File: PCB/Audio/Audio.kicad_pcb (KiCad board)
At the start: 2 copper layers, 70 x 70 mm, 54 parts, among them J1 Battery, J2 Reset, J3 TC2030-USB-NL-DS, J4 TF_PUSH, J5 USB-C-Socket-H, Q2 CJ2301, SW1 SW_Push, U1 R, U2 L, U3 TP4054, U4 ME6211C33M5G-N, U5 MAX98357A, U6 ESP32-S3-MINI-1

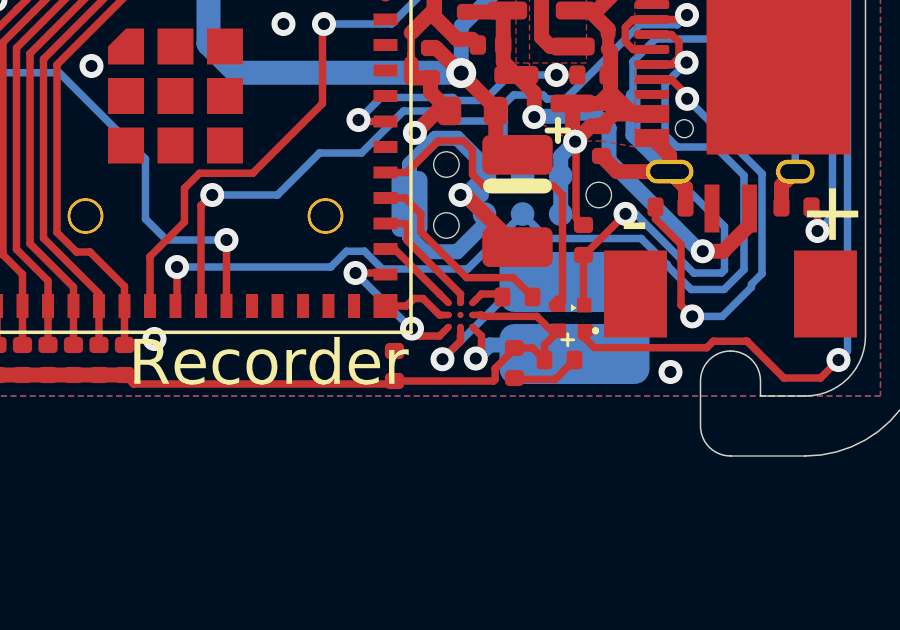
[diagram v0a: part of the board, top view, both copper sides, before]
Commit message: Tidy
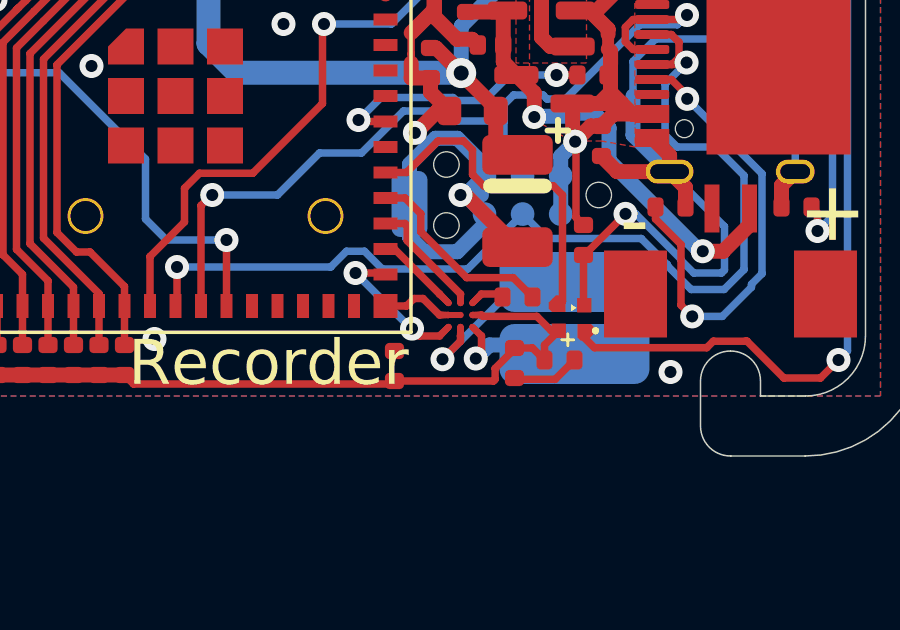
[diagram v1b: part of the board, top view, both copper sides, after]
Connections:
- U5 pad B2: unconnected-(U5-GAIN_SLOT-PadB2) -> GND
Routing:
- net GND: track 89.7 -> 90.4 mm
